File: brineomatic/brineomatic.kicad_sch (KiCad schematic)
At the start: 9 parts, among them U1 ESP32-S3-DEVKITC

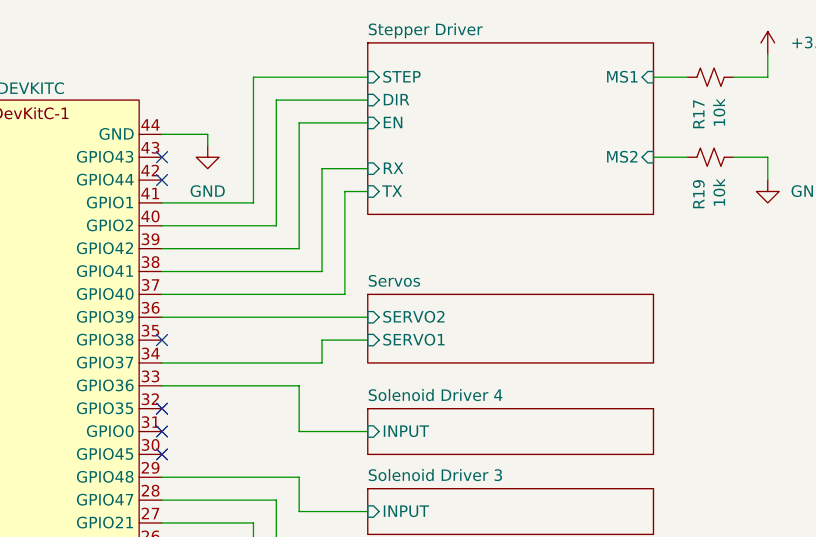
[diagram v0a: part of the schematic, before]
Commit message: worked on schematic and layout a bit more.
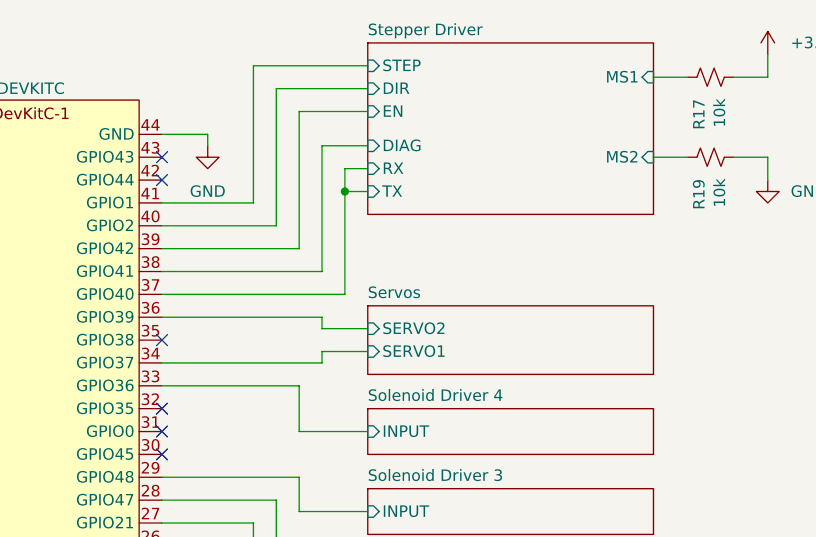
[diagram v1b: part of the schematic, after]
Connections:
- net Stepper Driver/TX is gone; now on net Stepper Driver/RX: U1.37 (GPIO40)
- net Stepper Driver/RX: no longer U1.38 (GPIO41)
- new net Stepper Driver/DIAG: U1.38 (GPIO41)
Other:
- sheet Stepper Driver ports: added DIAG; removed none
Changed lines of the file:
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@@
 	(paper "A4")
+	(junction
+		(at 219.71 57.15)
+		(diameter 0)
+		(color 0 0 0 0)
+	)
 	(junction
 		(at 39.37 142.24)
@@
 	(wire
 		(pts
-			(xy 209.55 44.45) (xy 222.25 44.45)
+			(xy 209.55 43.18) (xy 222.25 43.18)
 		)
 		(stroke
@@
 	(wire
 		(pts
-			(xy 217.17 73.66) (xy 222.25 73.66)
+			(xy 217.17 74.93) (xy 222.25 74.93)
 		)
 		(stroke
@@
 	(wire
 		(pts
+			(xy 222.25 54.61) (xy 219.71 54.61)
+		)
+		(stroke
+			(width 0)
+			(type default)
+		)
+	)
+	(wire
+		(pts
 			(xy 254 44.45) (xy 257.81 44.45)
 		)
@@
 	(wire
 		(pts
-			(xy 199.39 71.12) (xy 222.25 71.12)
+			(xy 217.17 72.39) (xy 222.25 72.39)
 		)
 		(stroke
@@
 	(wire
 		(pts
-			(xy 214.63 63.5) (xy 214.63 49.53)
+			(xy 214.63 63.5) (xy 214.63 48.26)
 		)
 		(stroke
@@
 	(wire
 		(pts
-			(xy 214.63 49.53) (xy 222.25 49.53)
+			(xy 214.63 48.26) (xy 222.25 48.26)
 		)
 		(stroke
@@
 	(wire
 		(pts
-			(xy 217.17 76.2) (xy 217.17 73.66)
+			(xy 217.17 76.2) (xy 217.17 74.93)
 		)
 		(stroke
@@
 	(wire
 		(pts
-			(xy 212.09 46.99) (xy 222.25 46.99)
+			(xy 212.09 45.72) (xy 222.25 45.72)
 		)
 		(stroke
@@
 	(wire
 		(pts
+			(xy 217.17 72.39) (xy 217.17 71.12)
+		)
+		(stroke
+			(width 0)
+			(type default)
+		)
+	)
+	(wire
+		(pts
 			(xy 209.55 93.98) (xy 209.55 110.49)
 		)
@@
 	(wire
 		(pts
-			(xy 209.55 58.42) (xy 209.55 44.45)
+			(xy 217.17 52.07) (xy 222.25 52.07)
+		)
+		(stroke
+			(width 0)
+			(type default)
+		)
+	)
+	(wire
+		(pts
+			(xy 209.55 58.42) (xy 209.55 43.18)
 		)
 		(stroke
@@
 	(wire
 		(pts
-			(xy 217.17 66.04) (xy 217.17 54.61)
+			(xy 217.17 52.07) (xy 217.17 66.04)
 		)
 		(stroke
@@
 	(wire
 		(pts
-			(xy 217.17 54.61) (xy 222.25 54.61)
-		)
-		(stroke
-			(width 0)
-			(type default)
-		)
-	)
-	(wire
-		(pts
 			(xy 180.34 114.3) (xy 201.93 114.3)
 		)
@@
 	(wire
 		(pts
-			(xy 212.09 60.96) (xy 212.09 46.99)
+			(xy 212.09 60.96) (xy 212.09 45.72)
 		)
 		(stroke
@@
 	(wire
 		(pts
+			(xy 217.17 71.12) (xy 199.39 71.12)
+		)
+		(stroke
+			(width 0)
+			(type default)
+		)
+	)
+	(wire
+		(pts
 			(xy 199.39 68.58) (xy 219.71 68.58)
 		)
@@
 		(pts
 			(xy 204.47 50.8) (xy 204.47 52.07)
+		)
+		(stroke
+			(width 0)
+			(type default)
+		)
+	)
+	(wire
+		(pts
+			(xy 219.71 54.61) (xy 219.71 57.15)
 		)
 		(stroke
@@
 	)
 	(sheet
-		(at 222.25 68.58)
+		(at 222.25 69.85)
 		(size 31.75 7.62)
 		(exclude_from_sim no)
@@
 		)
 		(property "Sheetname" "Servos"
-			(at 222.25 67.8684 0)
+			(at 222.25 69.1384 0)
 			(effects
 				(font
@@
 		)
 		(property "Sheetfile" "servo.kicad_sch"
-			(at 222.25 76.7846 0)
+			(at 222.25 78.0546 0)
 			(effects
 				(font
@@
 		)
 		(property "Field2" ""
-			(at 222.25 68.58 0)
+			(at 222.25 69.85 0)
 			(effects
 				(font
@@
 		)
 		(pin "SERVO1" input
-			(at 222.25 73.66 180)
+			(at 222.25 74.93 180)
 			(effects
 				(font
@@
 		)
 		(pin "SERVO2" input
-			(at 222.25 71.12 180)
+			(at 222.25 72.39 180)
 			(effects
 				(font
@@
 		)
 		(pin "DIR" input
-			(at 222.25 46.99 180)
+			(at 222.25 45.72 180)
 			(effects
 				(font
@@
 		)
 		(pin "EN" input
-			(at 222.25 49.53 180)
+			(at 222.25 48.26 180)
 			(effects
 				(font
@@
 		)
 		(pin "STEP" input
-			(at 222.25 44.45 180)
+			(at 222.25 43.18 180)
 			(effects
 				(font
@@
 			)
 		)
+		(pin "DIAG" input
+			(at 222.25 52.07 180)
+			(effects
+				(font
+					(size 1.27 1.27)
+				)
+				(justify left)
+			)
+		)

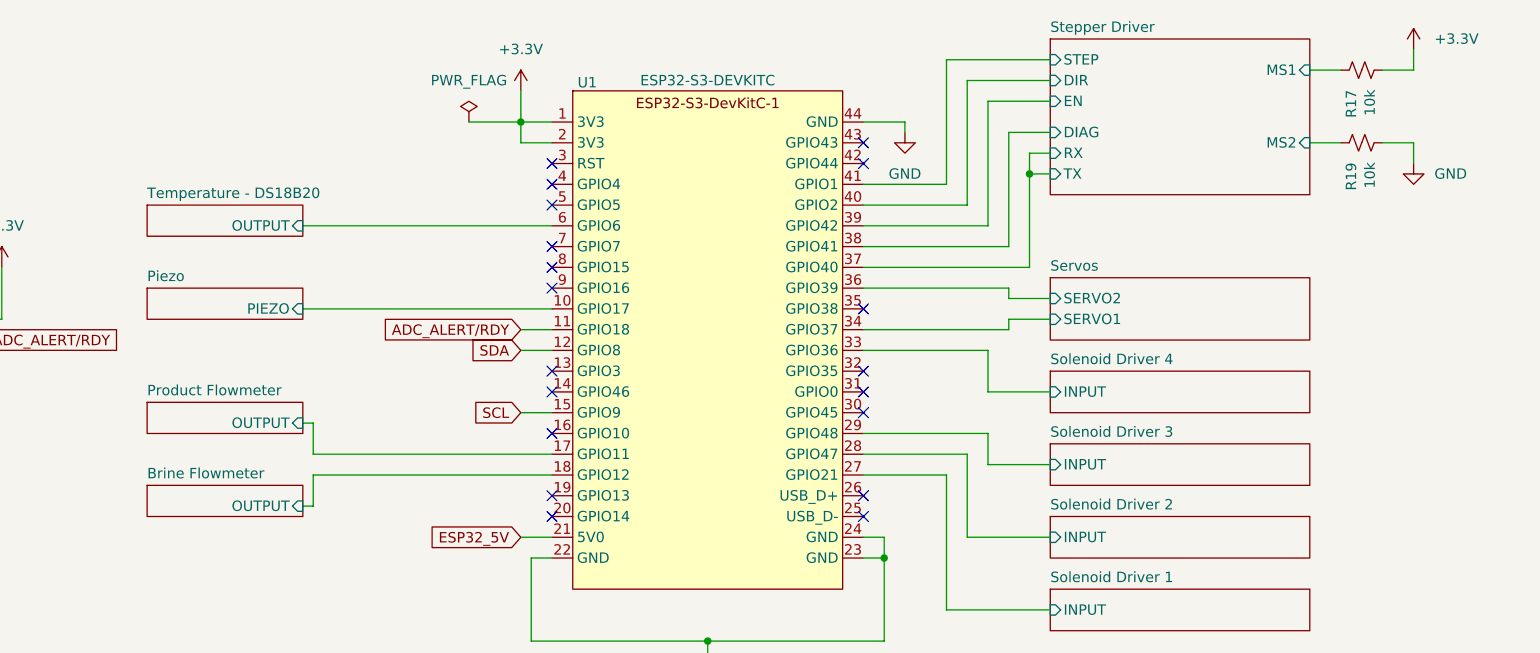
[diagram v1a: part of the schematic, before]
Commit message: lots of progress on Rev B
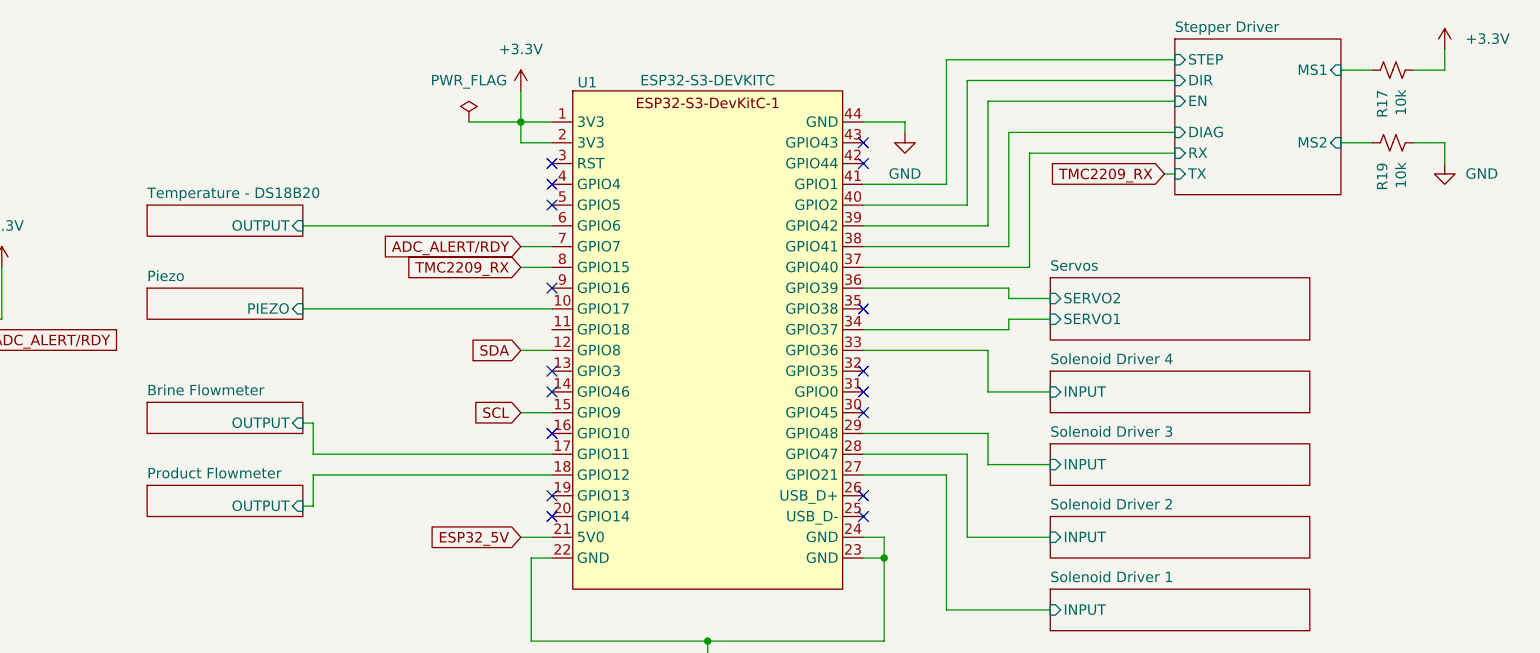
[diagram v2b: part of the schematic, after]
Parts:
- R17, R19: footprint (none) -> Resistor_SMD:R_0603_1608Metric
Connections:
- net ADC_ALERT/RDY: now also U1.7 (GPIO7); no longer U1.11 (GPIO18)
- net Brine Flowmeter/OUTPUT: now also U1.17 (GPIO11); no longer U1.18 (GPIO12)
- net Product Flowmeter/OUTPUT: now also U1.18 (GPIO12); no longer U1.17 (GPIO11)
- net TMC2209_RX: now reaches U1.8 (GPIO15)
- no-connect marks 19 -> 17
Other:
- moved on the sheet: R17, R19
